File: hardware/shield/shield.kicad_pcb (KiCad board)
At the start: 2 copper layers, 25.4 x 52.1 mm, 6 parts, among them J1 Conn_01x20, J2 Conn_01x20, J3 SEN0193, U1 TMP36

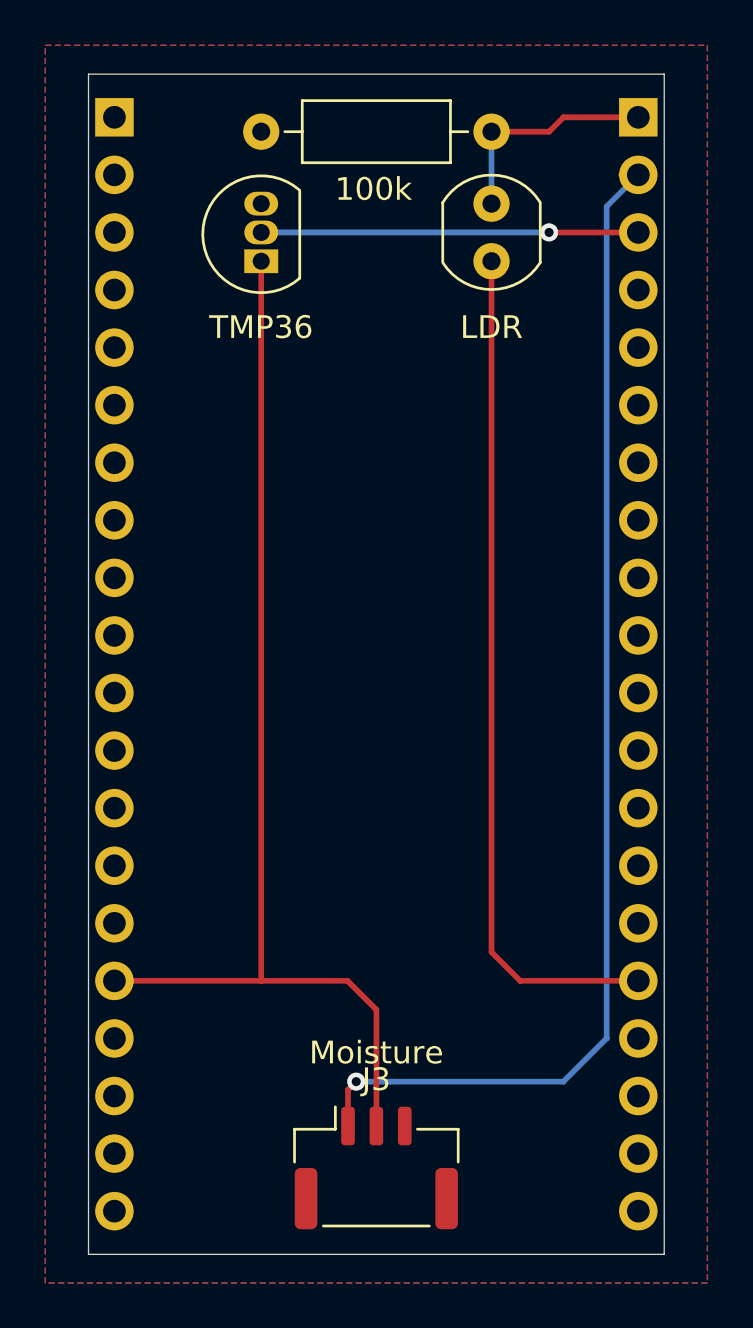
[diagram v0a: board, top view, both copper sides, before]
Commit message: updated pcb connector, added logo and version number
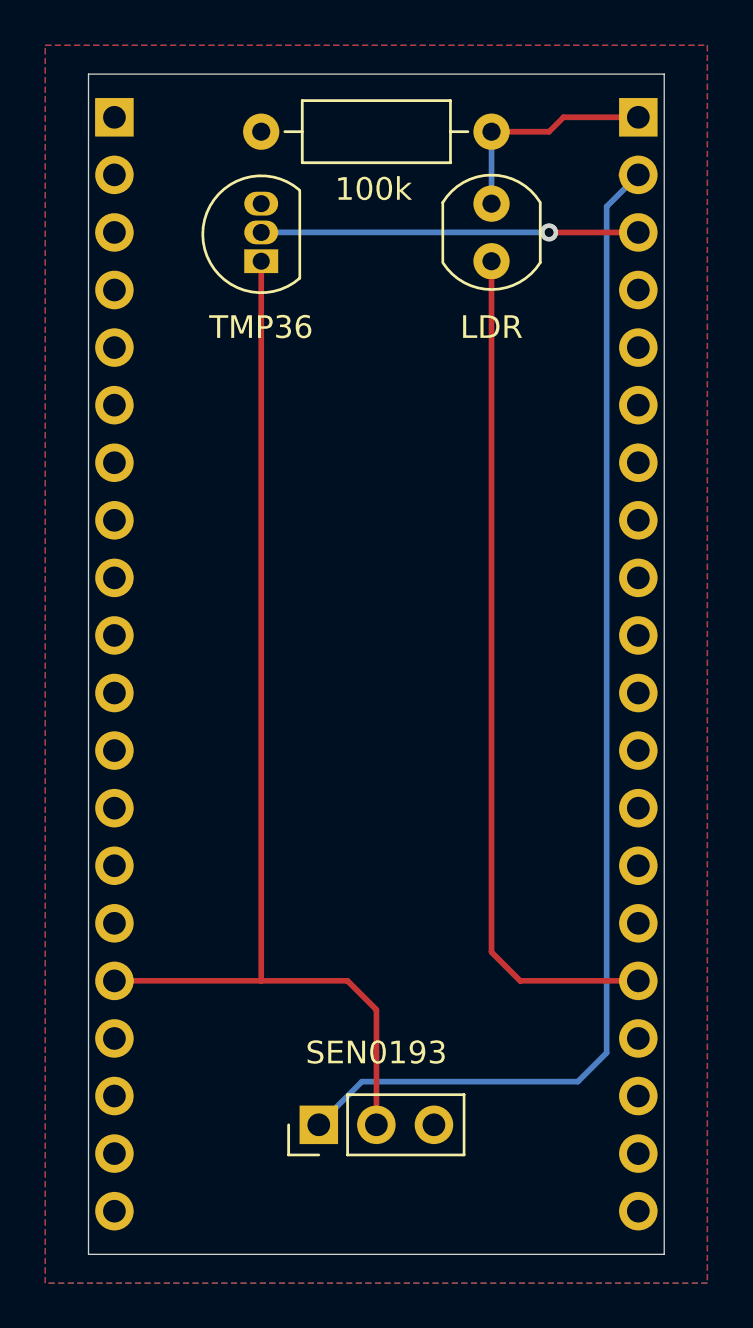
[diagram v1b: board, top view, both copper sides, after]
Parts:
- added G***: LOGO, healthyleaves:logo, F.Cu at (139.7, 111.8)
- J3: footprint Connector_JST:JST_GH_SM03B-GHS-TB_1x03-1MP_P1.25mm_Horizontal -> Connector_PinHeader_2.54mm:PinHeader_1x03_P2.54mm_Vertical
- moved J3 3.17 mm to (137.2, 122.6), turned to 90 degrees
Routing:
- net 37: track 53.4 -> 54.1 mm, vias 1 -> 0
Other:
- board text added: "HealthyLeaves ELEC/COEN 390 Project Team #2 201116DSJYKTTVBKN"
- board text added: "SEN0193"
- board text removed: "Moisture"

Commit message: Revert "Thomas object detection"
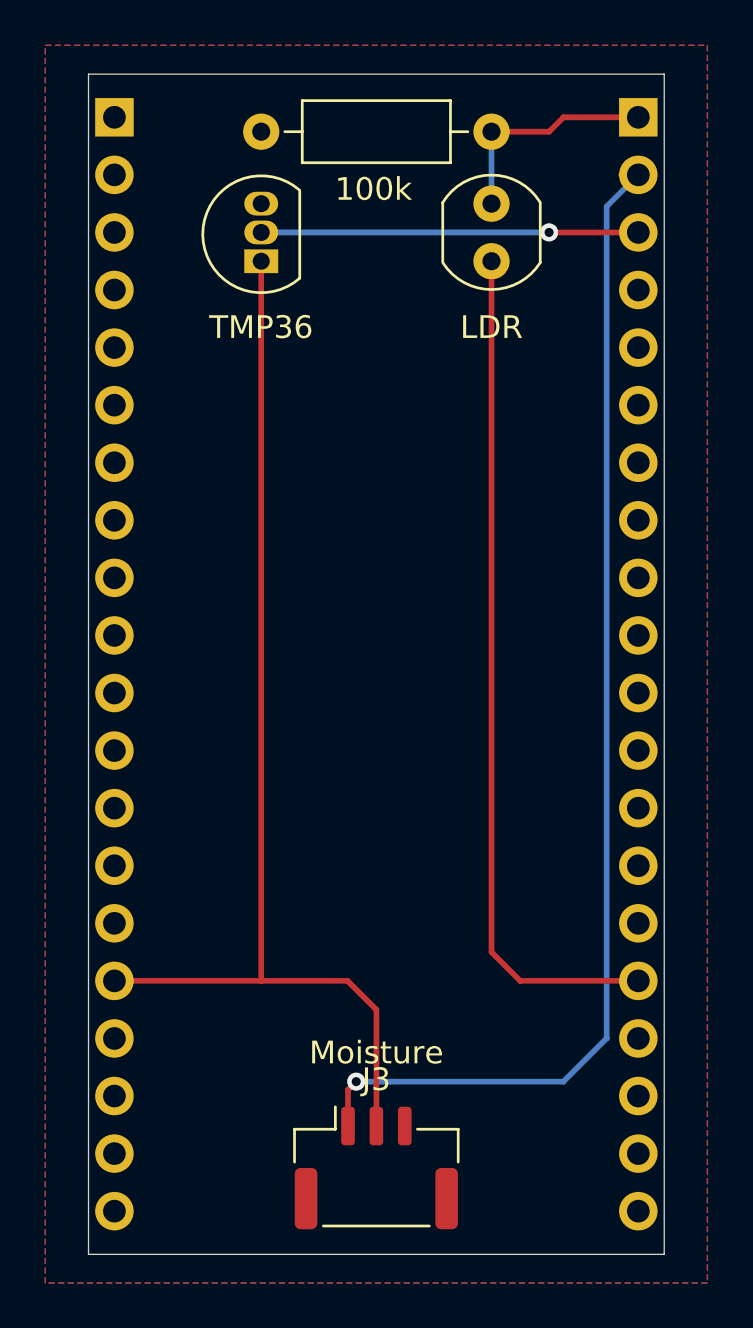
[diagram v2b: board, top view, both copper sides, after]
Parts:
- removed G***: LOGO, healthyleaves:logo
- J3: footprint Connector_PinHeader_2.54mm:PinHeader_1x03_P2.54mm_Vertical -> Connector_JST:JST_GH_SM03B-GHS-TB_1x03-1MP_P1.25mm_Horizontal
- moved J3 3.17 mm to (139.7, 124.5), turned to 0 degrees
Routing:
- net 37: track 54.1 -> 53.4 mm, vias 0 -> 1
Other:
- board text added: "Moisture"
- board text removed: "HealthyLeaves ELEC/COEN 390 Project Team #2 201116DSJYKTTVBKN"
- board text removed: "SEN0193"
